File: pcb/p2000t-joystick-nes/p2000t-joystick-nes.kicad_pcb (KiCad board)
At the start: 2 copper layers, 80 x 100 mm, 33 parts, among them J3 P2000T Port 2, SW1 KEYMAPPING, U1 74HC02, U2 74HC74, U3 74HC138, U4 74LS193, U5 74LS08, U6 SST39SF010, U7 SST39SF010, U8 74LS595, U9 74LS595, X1 1MHz

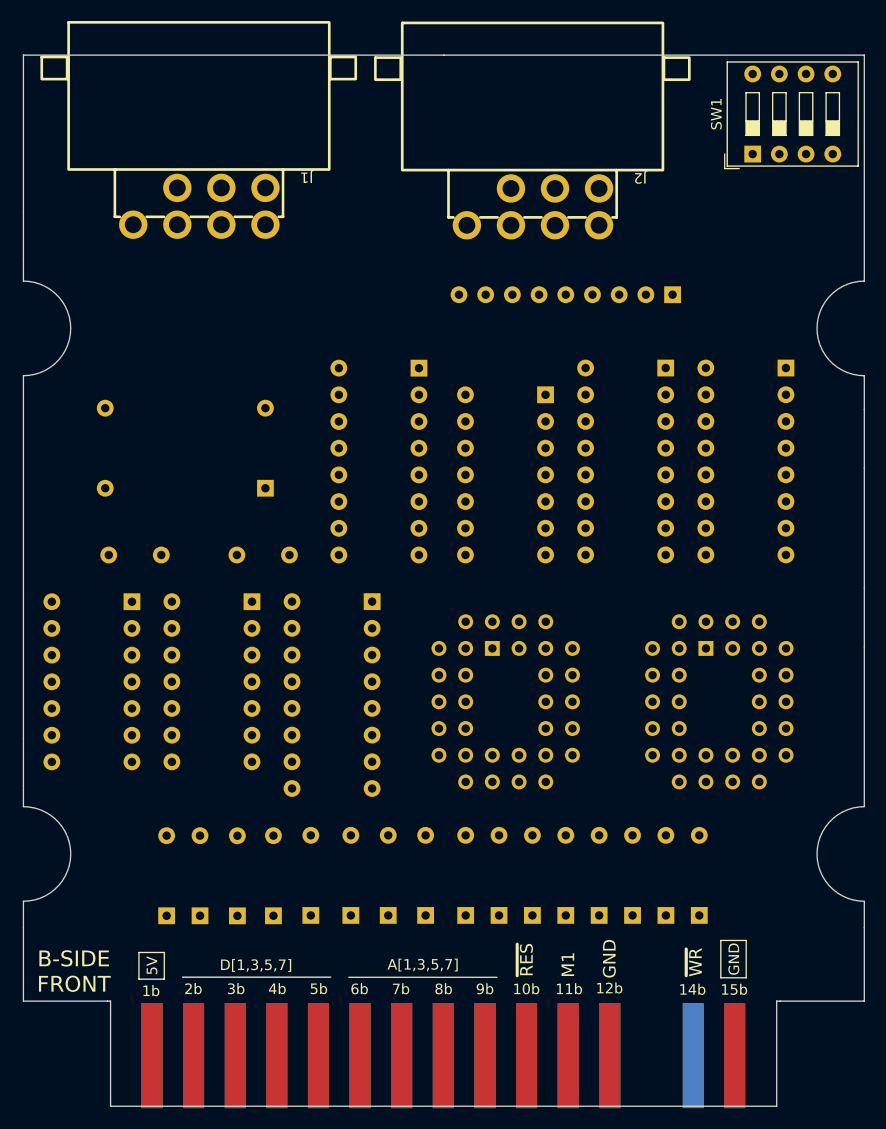
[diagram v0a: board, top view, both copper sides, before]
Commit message: Pre-routing commit
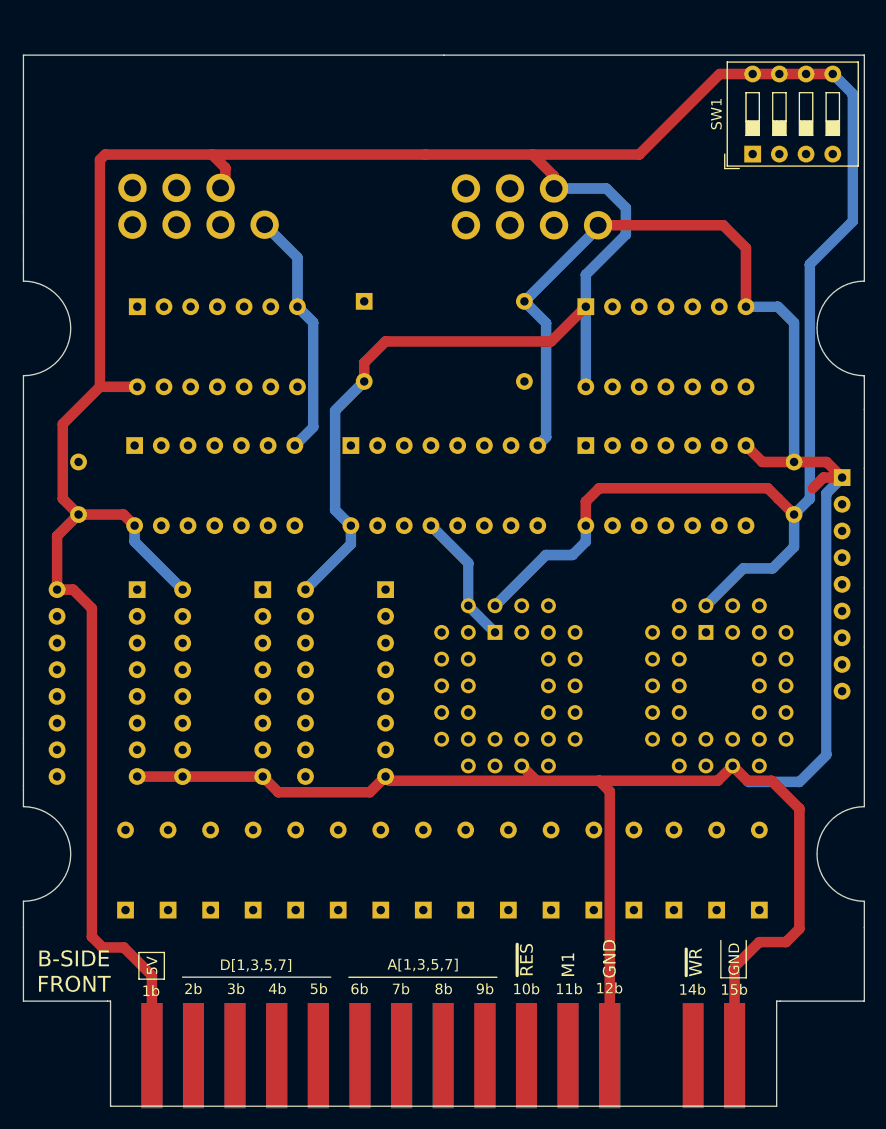
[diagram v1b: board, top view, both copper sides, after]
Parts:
- removed C3, C4: .1uF, Capacitor_THT:C_Disc_D5.0mm_W2.5mm_P5.00mm
- added C1: .1uF, Capacitor_THT:C_Disc_D5.0mm_W2.5mm_P5.00mm, B.Cu at (33.0, 69.8)
- added C2: .1uF, Capacitor_THT:C_Disc_D5.0mm_W2.5mm_P5.00mm, B.Cu at (101.1, 69.8)
- added U10: 74HC04, Package_DIP:DIP-14_W7.62mm_Socket, B.Cu at (38.6, 50.0)
- J1, J2, J3: moved to B.Cu
- moved U3 65.2 mm to (38.6, 77.0)
- moved U1 45.7 mm to (81.3, 63.2), turned to -90 degrees
- moved U2 42.4 mm to (81.3, 50.0), turned to -90 degrees
- moved U5 39.4 mm to (38.4, 63.2), turned to -90 degrees
- moved U9 30.8 mm to (58.9, 63.2), turned to -90 degrees
- moved D1 27.9 mm to (97.8, 107.4)
- moved U4 25.8 mm to (50.5, 77.0)
- moved RN1 23.7 mm to (105.7, 66.3), turned to -90 degrees
- moved D8 22.2 mm to (69.8, 107.4)
- moved D2 20.7 mm to (93.7, 107.4)
- moved X1 20.1 mm to (60.2, 49.5), turned to 0 degrees
- moved D7 15.0 mm to (73.9, 107.4)
- moved D3 13.5 mm to (89.7, 107.4)
- moved D6 7.76 mm to (78.0, 107.4)
- moved D4 6.50 mm to (85.9, 107.4)
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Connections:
- net Net-(U4-QA) renamed 500KHz
- J1 pad 2: CLK -> CTRLCLK
- J2 pad 2: CLK -> CTRLCLK
- U4 pad 5: CLK -> Net-(U4-UP)
- U4 pad 7: unconnected-(U4-QD-Pad7) -> Net-(U4-QD)
- U5 pad 10: CLK -> Net-(U5-Pad10)
- U5 pad 4: Net-(U5-Pad3) -> Net-(U4-QC)
- U5 pad 5: Net-(U4-QC) -> Net-(U4-QD)
- U5 pad 6: Net-(U5-Pad6) -> Net-(U5-Pad10)
- U5 pad 9: Net-(U5-Pad6) -> Net-(U5-Pad3)
- X1 pad 8: CLK -> Net-(U4-UP)
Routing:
- net VCC: track 0.00 -> 362.1 mm
- net GND: track 0.00 -> 274.4 mm
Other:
- board text added: "jlcjlcjlcjlc"
